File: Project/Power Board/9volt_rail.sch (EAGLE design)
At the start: 54 parts, among them IC1 TL331, Q1 BSS84, Q2 BSS123

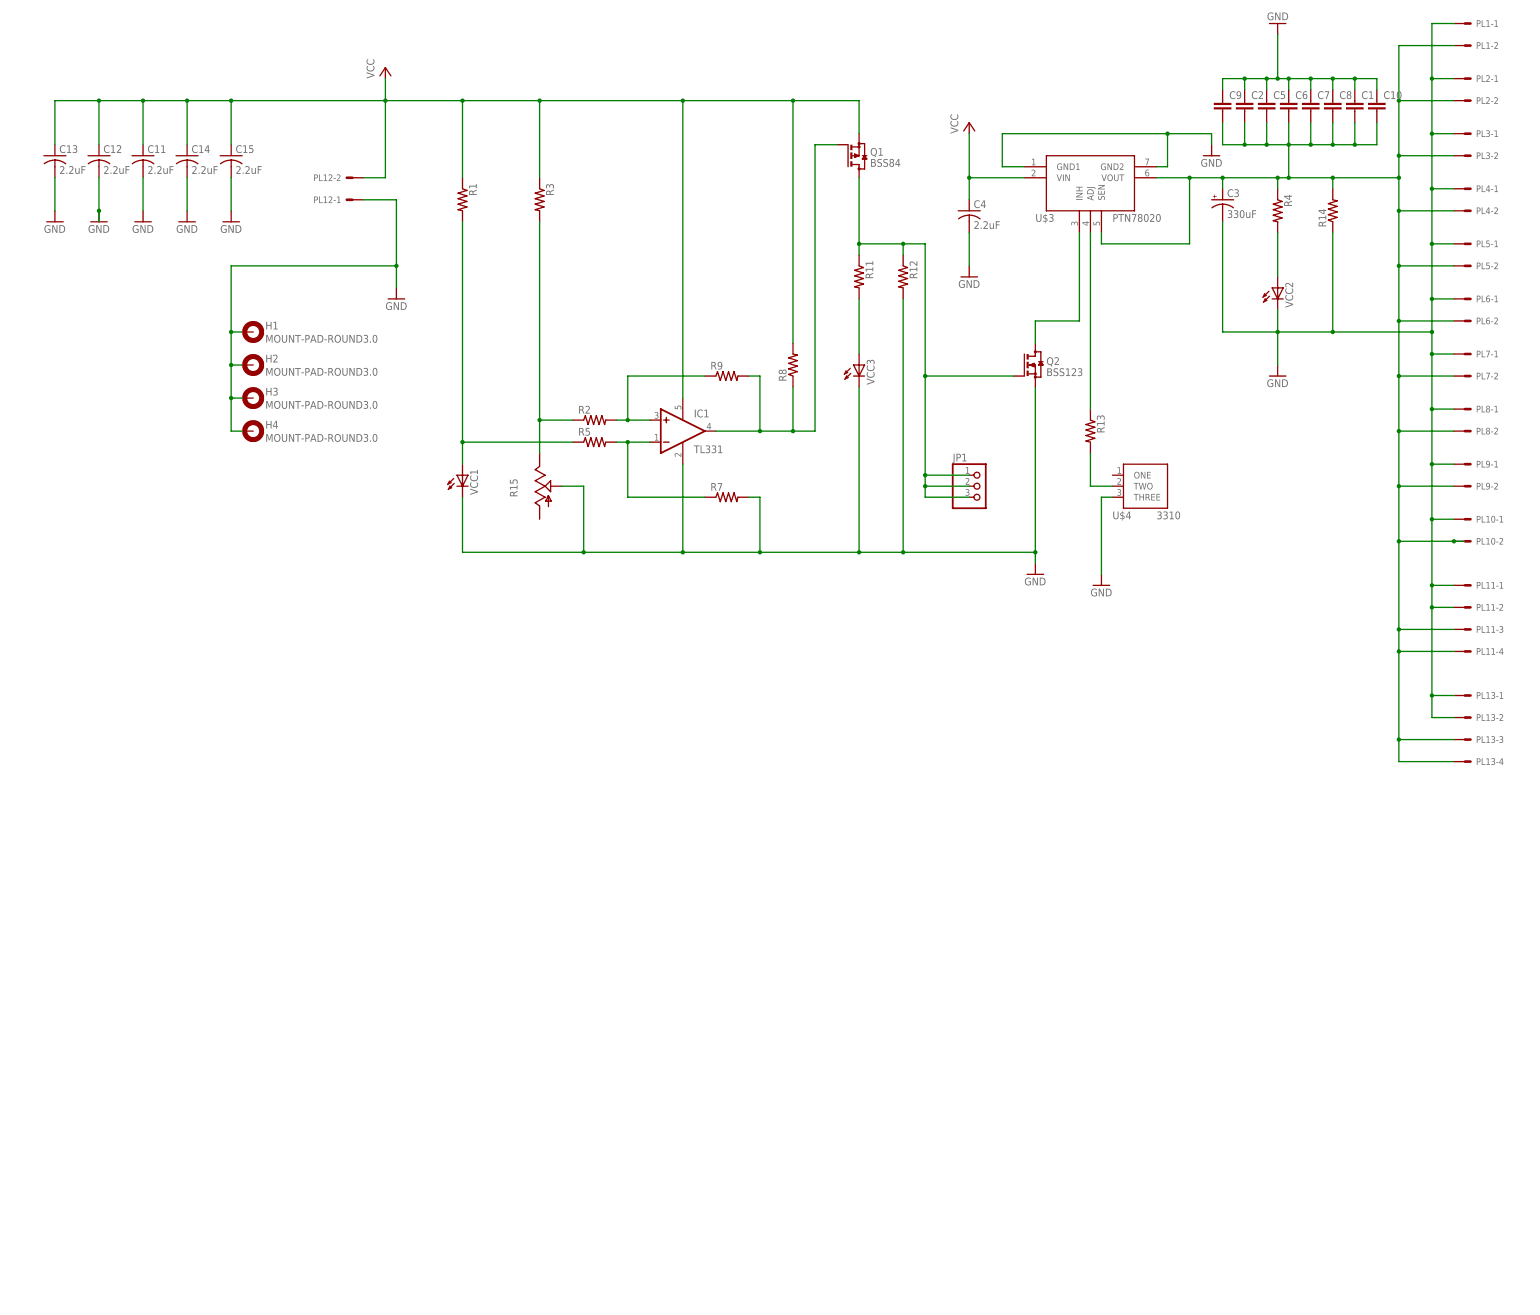
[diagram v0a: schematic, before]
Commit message: update
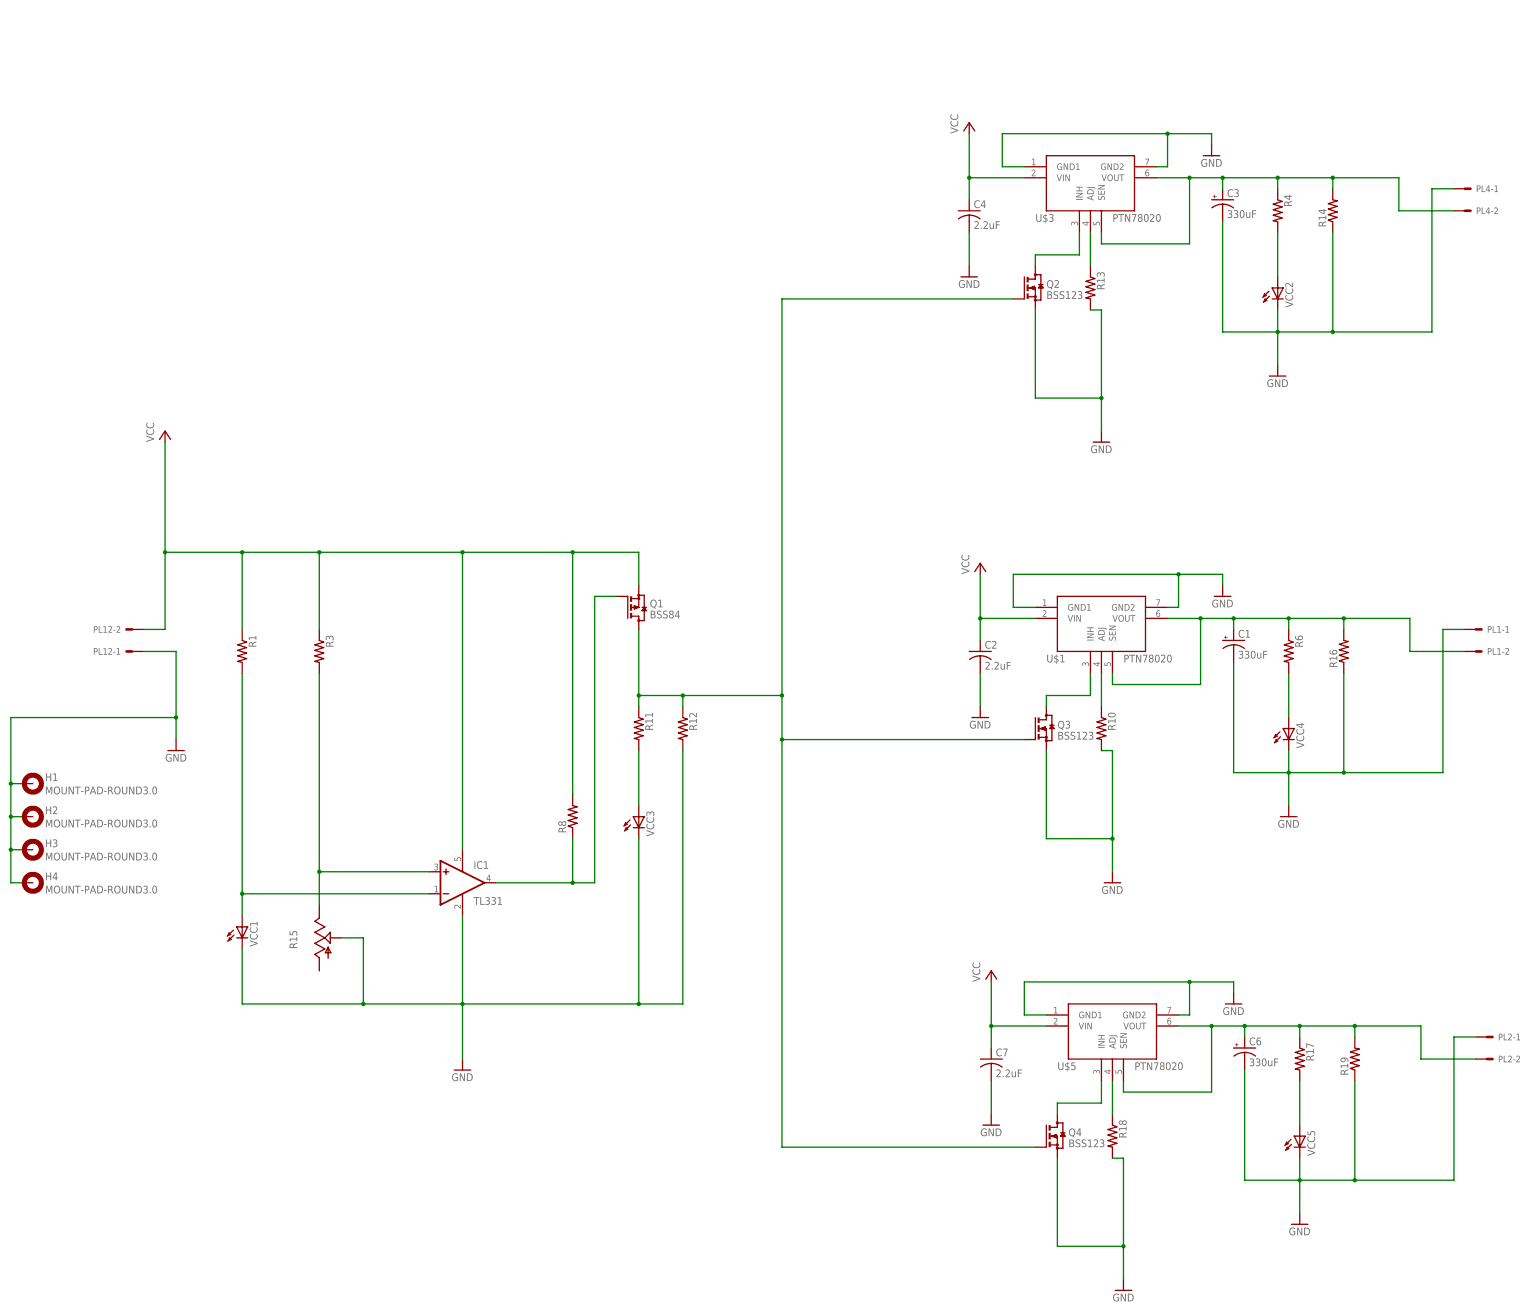
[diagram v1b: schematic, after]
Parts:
- removed C10, C5, C8, C9: (no value), rcl:C-EUC0805
- removed C11, C12, C13, C14, C15: 2.2uF, adafruit:C-USC0805
- removed JP1: (no value), adafruit:PINHD-1X3
- removed PL10, PL3, PL5, PL6, PL7, PL8, PL9: (no value), con-molex-2:555X-2H
- removed PL11, PL13: (no value), con-molex-2:555X-4H
- removed R2, R5, R7, R9: (no value), adafruit:R-US_M0805
- removed U$4: 3310-001, 3310-001:3310-001
- added Q3, Q4: BSS123, transistor-small-signal:BSS123
- added R10, R17, R18, R6: (no value), adafruit:R-US_M0805
- added R16, R19: (no value), resistor:R-US_0617/17
- added U$1, U$5: PTH78020-SMD, PTN78020:PTH78020-SMD
- added VCC4, VCC5: (no value), adafruit:LED5MM
- C1, C6: value (none) -> 330uF; device rcl:C-EUC0805 -> rcl:CPOL-USE5-10.5
- C2, C7: value (none) -> 2.2uF; device rcl:C-EUC0805 -> adafruit:C-USC0805
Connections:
- removed net N$1: R13.2, U$4.TWO
- removed net N$3: R1.2, R5.1, VCC1.A
- removed net N$5: JP1.1, JP1.2, JP1.3, Q1.D, Q2.G, R11.1, R12.1
- removed net N$6: R15.E, R2.1, R3.2
- new net N$14: R6.2, VCC4.A
- new net N$15: C1.+, PL1-2.S, R16.2, R6.1, U$1.SEN, U$1.VOUT
- new net N$16: R10.1, U$1.ADJ
- new net N$18: Q3.D, U$1.INH
- new net N$19: R17.2, VCC5.A
- new net N$20: C6.+, PL2-2.S, R17.1, R19.2, U$5.SEN, U$5.VOUT
- new net N$21: R18.1, U$5.ADJ
- new net N$23: Q4.D, U$5.INH
- new net N$24: Q1.D, Q2.G, Q3.G, Q4.G, R11.1, R12.1
- net GND: now also C1.-, C2.2, C6.-, C7.2, Q3.S, Q4.S, R10.2, R13.2, R16.1, R18.2, R19.1, U$1.GND1, U$1.GND2, U$5.GND1, U$5.GND2, VCC4.C, VCC5.C; no longer C1.1, C10.1, C11.2, C12.2, C13.2, C14.2, C15.2, C2.1, C5.1, C6.1, C7.1, C8.1, C9.1, PL10-1.S, PL11-1.S, PL11-2.S, PL13-1.S, PL13-2.S, PL3-1.S, PL5-1.S, PL6-1.S, PL7-1.S, PL8-1.S, PL9-1.S, R7.2, U$4.THREE
- net N$11: no longer C1.2, C10.2, C2.2, C5.2, C6.2, C7.2, C8.2, C9.2, PL1-2.S, PL10-2.S, PL11-3.S, PL11-4.S, PL13-3.S, PL13-4.S, PL2-2.S, PL3-2.S, PL5-2.S, PL6-2.S, PL7-2.S, PL8-2.S, PL9-2.S
- net N$2: no longer R9.2
- net N$4: now also R15.E, R3.2; no longer R2.2, R9.1
- net N$7: now also R1.2, VCC1.A; no longer R5.2, R7.1
- net VCC: now also C2.1, C7.1, U$1.VIN, U$5.VIN; no longer C11.1, C12.1, C13.1, C14.1, C15.1
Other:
- moved on the sheet: C2, C7, H1, H2, H3, H4, IC1, PL1-1, PL1-2, PL12-1, PL12-2, PL2-1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
